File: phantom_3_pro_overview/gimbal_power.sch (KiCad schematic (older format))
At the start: 1 part

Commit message: Overview: Upgraded to KiCAD 5.0.1.
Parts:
- U?: symbol IC_DIL8 -> ic_dil_generic:IC_DIL8
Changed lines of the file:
@@
-EESchema Schematic File Version 2
-LIBS:power
-LIBS:device
-LIBS:transistors
-LIBS:conn
-LIBS:linear
-LIBS:regul
-LIBS:74xx
-LIBS:cmos4000
-LIBS:adc-dac
-LIBS:memory
-LIBS:xilinx
-LIBS:microcontrollers
-LIBS:dsp
-LIBS:microchip
-LIBS:analog_switches
-LIBS:motorola
-LIBS:texas
-LIBS:intel
-LIBS:audio
-LIBS:interface
-LIBS:digital-audio
-LIBS:philips
-LIBS:display
-LIBS:cypress
-LIBS:siliconi
-LIBS:opto
-LIBS:atmel
-LIBS:contrib
-LIBS:valves
-LIBS:motors
-LIBS:ic_dil_generic
-LIBS:sensors
-LIBS:u-blox
-LIBS:amplifiers
-LIBS:transistors-switches
-LIBS:transistors-power
-LIBS:sensors-v2
-LIBS:regul-v2
+EESchema Schematic File Version 4
 LIBS:phantom_3_pro_overview-cache
-EELAYER 25 0
+EELAYER 26 0
 EELAYER END
 $Descr A4 11693 8268
@@
 RIBBON_CENTER
 $Comp
-L IC_DIL8 U?
+L ic_dil_generic:IC_DIL8 U?
 U 1 1 5A1F3EFF
 P 1150 800

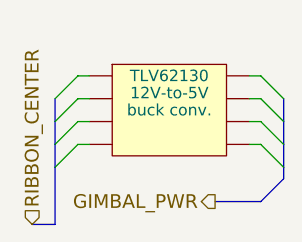
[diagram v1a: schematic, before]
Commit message: All: Finished updating to KiCad 5.0.1.
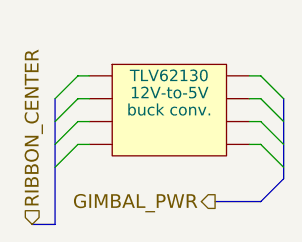
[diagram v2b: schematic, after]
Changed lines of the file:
@@
 	800  950  750  950
 Wire Bus Line
-	650  750  650  850
-Wire Bus Line
-	650  850  650  950
-Wire Bus Line
-	650  950  650  1050
-Wire Bus Line
-	650  1050 650  1300
-Wire Bus Line
 	650  1300 550  1300
-Wire Bus Line
-	1650 1100 1650 1050
-Wire Bus Line
-	1650 1050 1650 950
-Wire Bus Line
-	1650 950  1650 850
-Wire Bus Line
-	1650 850  1650 750
 Text HLabel 1350 1200 0    60   Output ~ 0
 GIMBAL_PWR
@@
 Wire Bus Line
 	1550 1200 1350 1200
+Wire Bus Line
+	650  750  650  1300
+Wire Bus Line
+	1650 750  1650 1100
 $EndSCHEMATC
